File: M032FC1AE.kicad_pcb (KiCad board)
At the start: 2 copper layers, 35 parts, among them IC1 M032FC1AE, J1 Conn_01x10, J2 Conn_01x03, J4 USB_C_Receptacle_USB2.0_16P, J5 Conn_01x03, J6 Conn_01x05, J7 Conn_02x08_Odd_Even, Q1 S8050, SW1 SW_Push, SW2 SW_Push, U1 AMS1117-1.8, U2 AMS1117-3.3, U3 USBLC6-2SC6

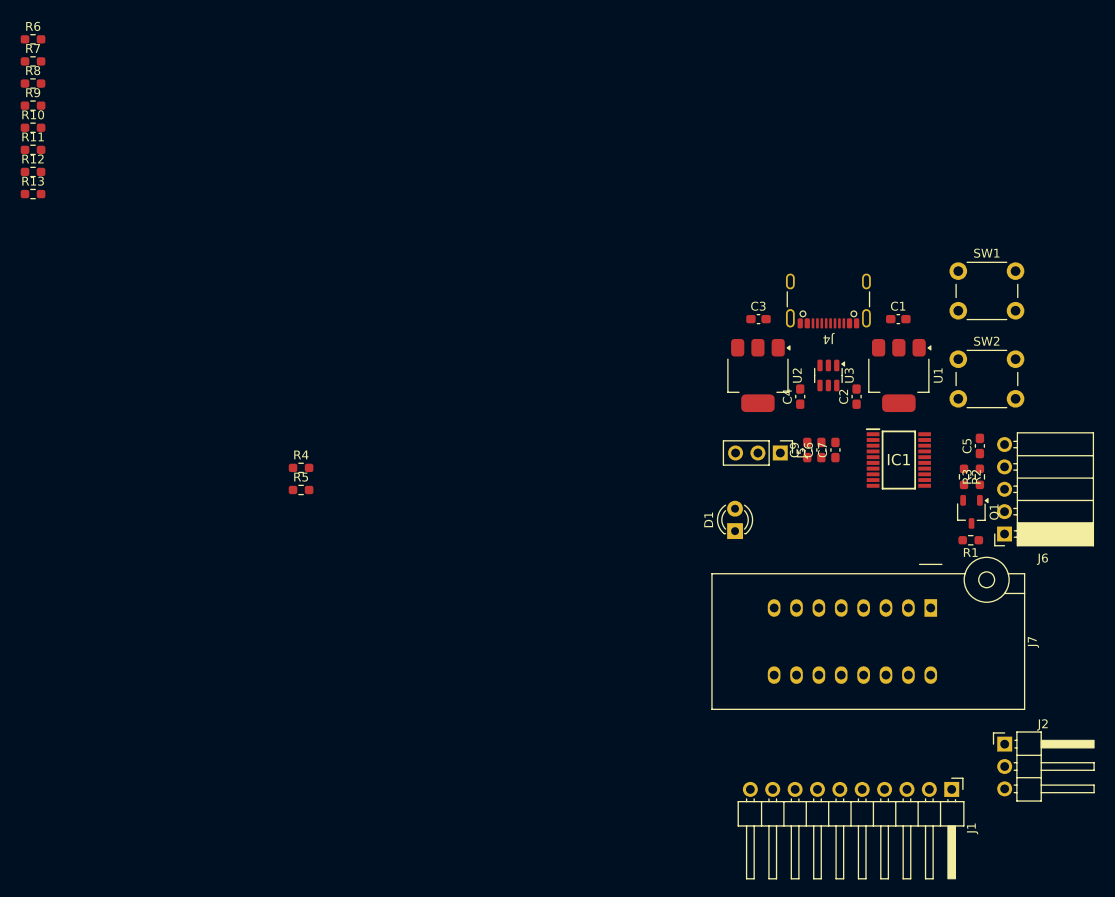
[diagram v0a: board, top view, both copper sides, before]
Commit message: ffffddd
Change-Id: I1eeee01593b08b9acbec1eab3a106692ce76c6c6
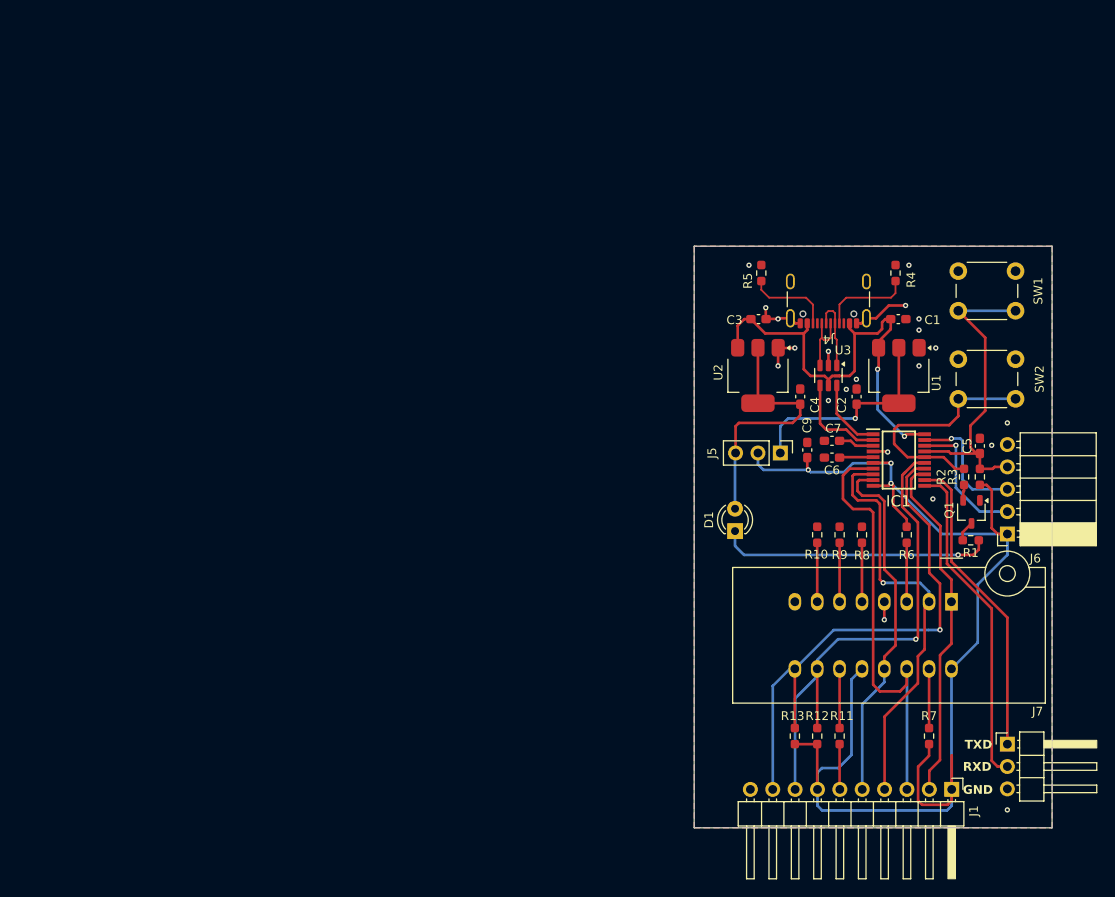
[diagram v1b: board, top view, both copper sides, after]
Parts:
- J7: value Conn_02x08_Odd_Even -> Conn_02x08_Counter_Clockwise
- moved R7 127.4 mm to (171.6, 112.7), turned to -90 degrees
- moved R6 114.0 mm to (169.1, 89.9), turned to -90 degrees
- moved R11 113.2 mm to (161.5, 112.7), turned to -90 degrees
- moved R12 109.7 mm to (158.9, 112.7), turned to 90 degrees
- moved R8 107.2 mm to (164.0, 89.9), turned to -90 degrees
- moved R13 106.2 mm to (156.4, 112.7), turned to 90 degrees
- moved R9 103.7 mm to (161.5, 89.9), turned to -90 degrees
- moved R10 100.3 mm to (158.9, 89.9), turned to -90 degrees
- moved R4 71.0 mm to (167.8, 60.2), turned to 90 degrees
- moved R5 57.8 mm to (152.6, 60.2), turned to 90 degrees
- moved J7 2.45 mm to (174.2, 97.5)
- moved C6 1.48 mm to (160.6, 81.1), turned to 180 degrees
- moved C7 1.12 mm to (160.6, 79.2), turned to 180 degrees
- moved J6 0.32 mm to (180.5, 89.8)
- moved J2 0.31 mm to (180.5, 113.7)
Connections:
- J1 pad 8: isci1_clk -> usci1_clk
- J7 pad 10: VCC -> usci1_clk
- J7 pad 12: Net-(J7-Pin_12) -> VCC
- J7 pad 13: Net-(J7-Pin_13) -> spi_mosi
- J7 pad 14: usci1_clk -> spi_clk
- J7 pad 15: GND -> Net-(J7-Pin_15)
- J7 pad 16: usci1_data -> VCC
- J7 pad 2: VCC -> spi_miso
- J7 pad 3: spi_miso -> Net-(J7-Pin_3)
- J7 pad 4: Net-(J7-Pin_4) -> GND
- J7 pad 6: spi_clk -> Net-(J7-Pin_6)
- J7 pad 7: GND -> Net-(J7-Pin_7)
- J7 pad 8: spi_mosi -> GND
- J7 pad 9: Net-(J7-Pin_9) -> usci1_data
- R10 pad 2: Net-(J7-Pin_13) -> Net-(J7-Pin_7)
- R11 pad 1: Net-(J7-Pin_12) -> Net-(J7-Pin_11)
- R6 pad 2: Net-(J7-Pin_5) -> Net-(J7-Pin_3)
- R7 pad 1: Net-(J7-Pin_4) -> Net-(J7-Pin_15)
- R8 pad 2: Net-(J7-Pin_9) -> Net-(J7-Pin_5)
- R9 pad 2: Net-(J7-Pin_11) -> Net-(J7-Pin_6)
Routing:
- net VCC: track 0.00 -> 146.4 mm, vias 0 -> 3
- net usci1_data: track 0.00 -> 61.4 mm, vias 0 -> 1
- net usci1_clk: track 0.00 -> 57.5 mm, vias 0 -> 1
- net VBUS: track 0.00 -> 52.1 mm, vias 0 -> 2
- net spi_clk: track 0.00 -> 50.0 mm
- net spi_miso: track 0.00 -> 47.4 mm, vias 0 -> 1
- net spi_mosi: track 0.00 -> 41.2 mm
- net spi_ss: track 0.00 -> 39.9 mm
- net uart_tx: track 0.00 -> 37.5 mm
- net rst: track 0.00 -> 36.7 mm
- net uart_rx: track 0.00 -> 35.0 mm
- net Net-(D1-K): track 0.00 -> 31.1 mm, vias 0 -> 1
- net +3.3V: track 0.00 -> 29.7 mm
- net ISP: track 0.00 -> 27.1 mm
- net GND: track 0.00 -> 26.3 mm, vias 0 -> 21
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- added copper zone on B.Cu, net GND
- added copper zone on F.Cu, net GND
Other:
- board outline added: 40.6 x 66 mm
- board text added: "GND"
- board text added: "I2C_CLK"
- board text added: "I2C_DAT"
- board text added: "RXD"
- board text added: "SPI_CLK"
- board text added: "SPI_MISO"
- board text added: "SPI_MOSI"
- board text added: "SPI_SS"
- board text added: "TXD"
- board text added: "VCC"
